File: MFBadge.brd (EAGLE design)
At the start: 88.9 x 50.8 mm, 0 parts

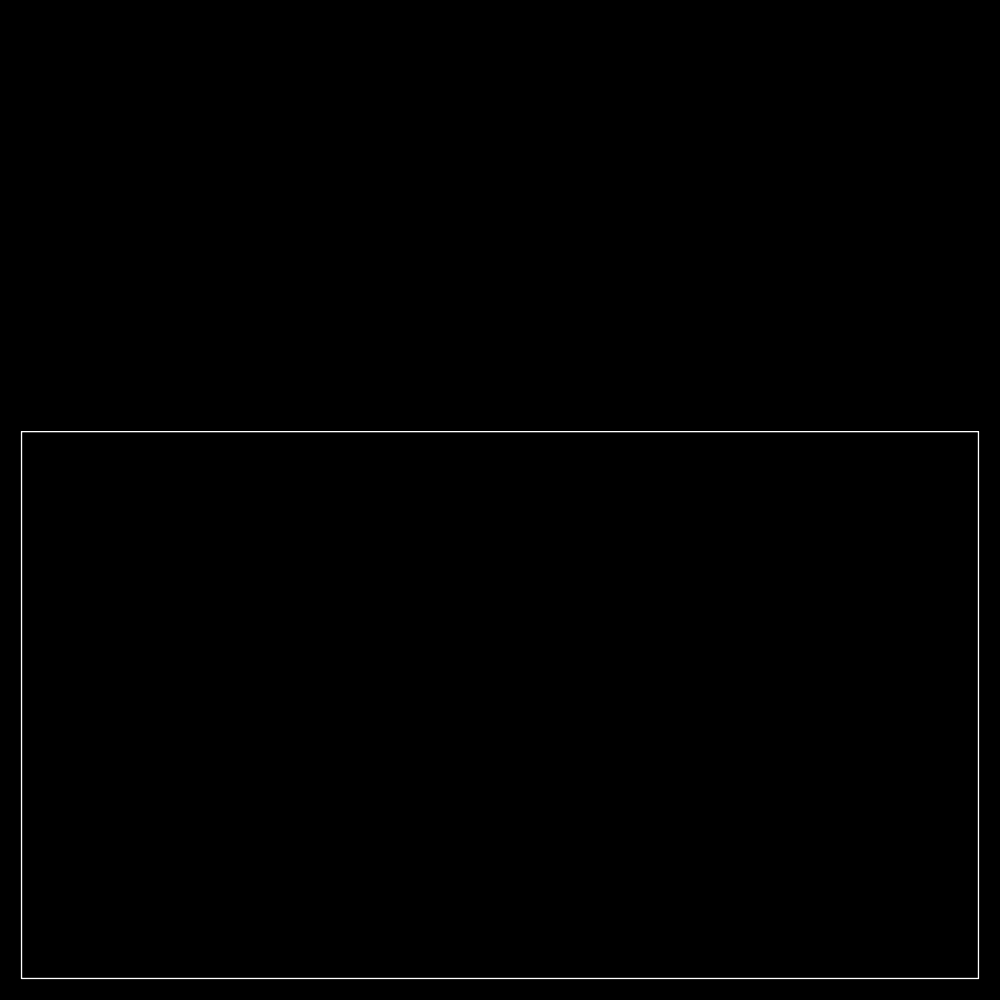
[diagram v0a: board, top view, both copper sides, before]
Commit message: Added images. Checking in todays work.
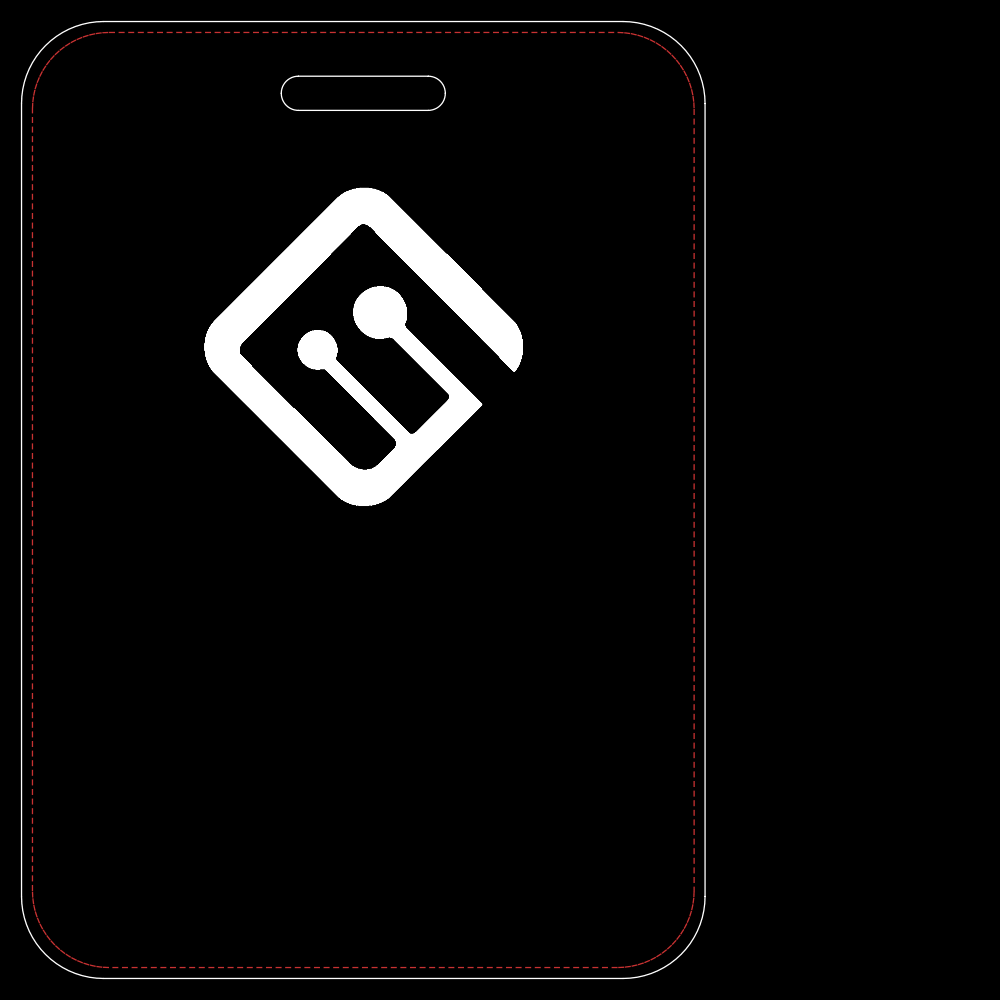
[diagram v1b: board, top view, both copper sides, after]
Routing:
- added copper zone on layer 1, net N$1
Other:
- board size 88.9 x 50.8 mm -> 63.5 x 88.9 mm
